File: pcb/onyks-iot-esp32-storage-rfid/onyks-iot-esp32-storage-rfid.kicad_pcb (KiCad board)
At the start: 4 copper layers, 79.5 x 45.5 mm, 22 parts, among them J1 Conn_01x02_Pin, J2 Conn_01x06_Pin, J3 Conn_02x05_Top_Bottom, J5 Conn_01x03_Pin, J6 Conn_01x01_Pin, Q1 SS8050, Q2 SS8050, SW3 SW_Push, SW4 SW_Push, U1 ESP32-WROOM-32D, U2 TLV75733PDBV

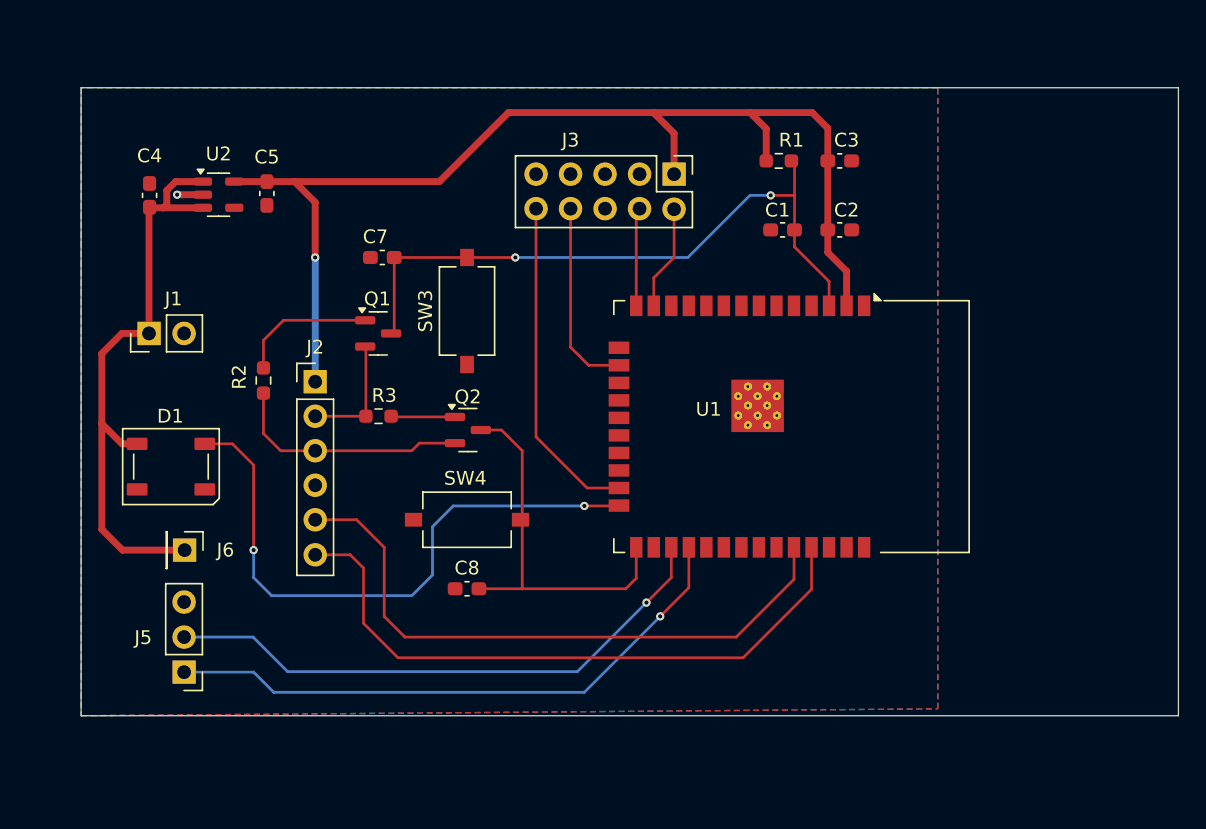
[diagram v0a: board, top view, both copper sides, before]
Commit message: PCB gotowe do review
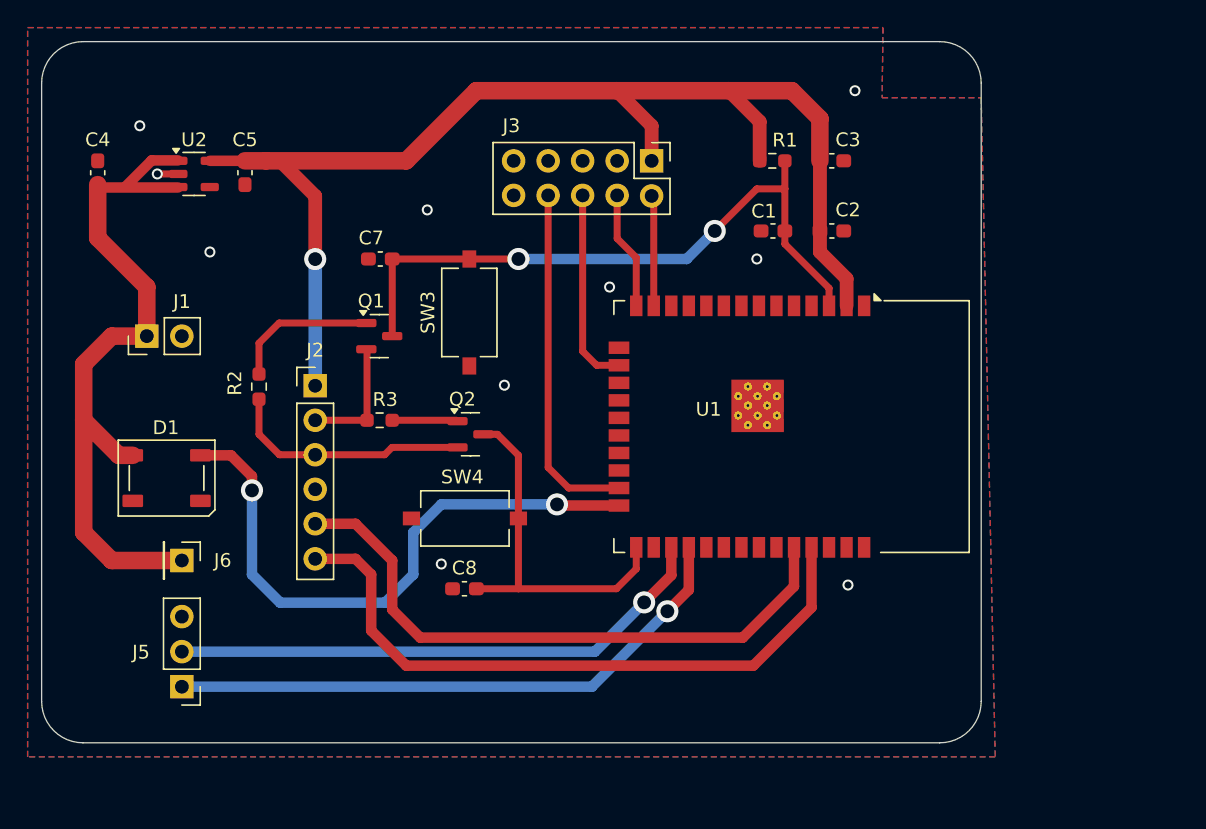
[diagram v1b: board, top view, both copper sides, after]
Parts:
- moved C4 4.10 mm to (110.7, 95.9)
- moved U2 2.33 mm to (117.7, 95.9)
- moved C5 2.19 mm to (121.4, 95.9)
- moved J3 1.89 mm to (150.9, 95.0)
- moved J5 1.07 mm to (116.8, 133.1)
- moved D1 0.89 mm to (115.7, 118.0)
- moved J6 0.78 mm to (116.8, 124.0)
- moved C1 0.70 mm to (159.7, 100.1)
- moved C2 0.57 mm to (163.9, 100.1)
- moved C3 0.57 mm to (163.9, 95.0)
- moved R2 0.55 mm to (122.4, 111.4)
- moved R1 0.47 mm to (159.6, 95.0)
- moved Q2 0.36 mm to (137.7, 114.8)
- moved R3 0.30 mm to (131.2, 113.8)
- moved J2 0.29 mm to (126.5, 111.3)
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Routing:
- net VCC: track 43.7 -> 52.8 mm
- net VDD33: track 83.2 -> 92.0 mm
- net /ESP32/RXD: track 41.4 -> 39.8 mm
- net /ESP32/MTDI: track 7.14 -> 8.57 mm
- net /ESP32/MTDO: track 24.1 -> 25.5 mm
- net /ESP32/PROGRAM_TXD: track 46.5 -> 47.6 mm
- net /ESP32/IO0: track 27.4 -> 26.6 mm
- net Net-(Q1-B): track 9.98 -> 10.6 mm
- net /ESP32/PROGRAM_RXD: track 45.2 -> 44.6 mm
- net /ESP32/TXD: track 43.2 -> 42.7 mm
- net /ESP32/EN: track 47.5 -> 48.0 mm
- net GND: track 1.86 -> 1.53 mm, vias 1 -> 10
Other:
- board size 79.5 x 45.5 mm -> 68.1 x 50.8 mm

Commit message: projekt PCB v2
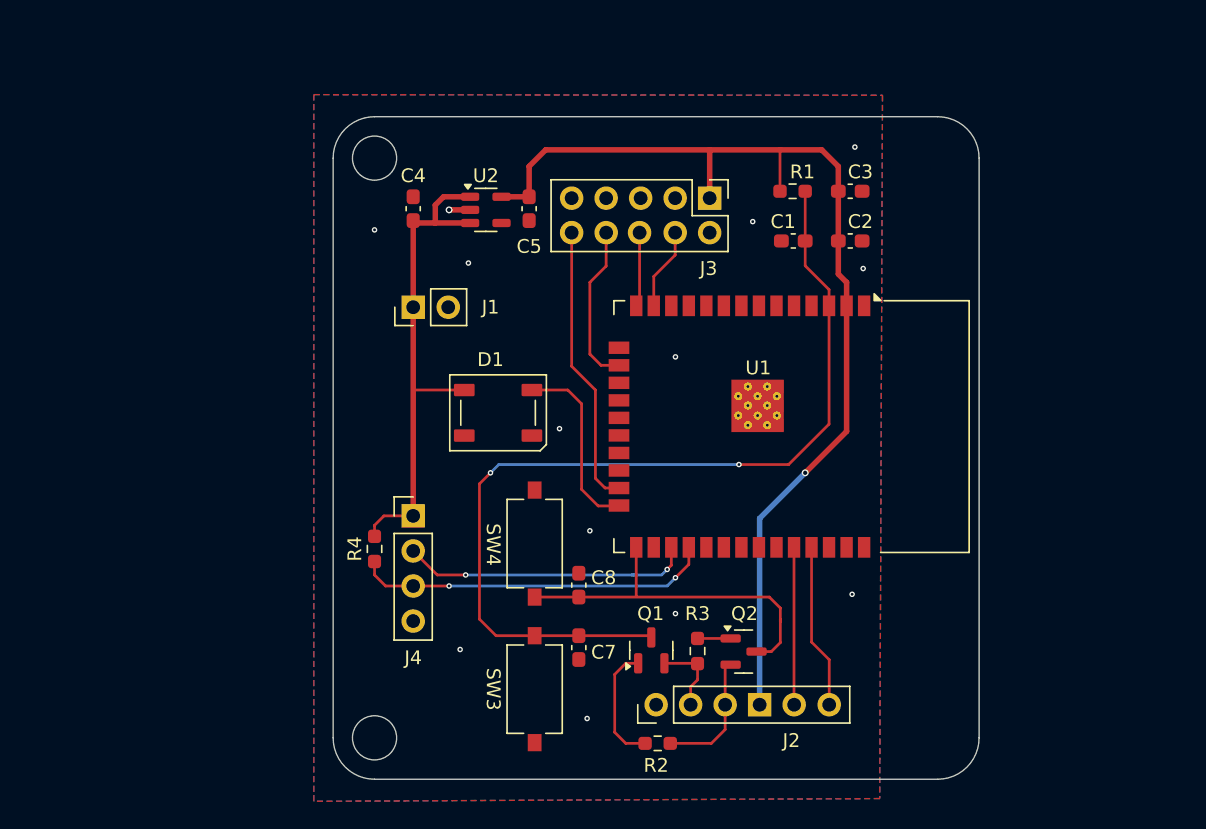
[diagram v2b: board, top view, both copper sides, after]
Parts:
- removed J5: Conn_01x03_Pin, Connector_PinHeader_2.54mm:PinHeader_1x03_P2.54mm_Vertical
- removed J6: Conn_01x01_Pin, Connector_PinHeader_2.54mm:PinHeader_1x01_P2.54mm_Vertical
- added J4: Conn_01x04_Pin, Connector_PinHeader_2.54mm:PinHeader_1x04_P2.54mm_Vertical, F.Cu at (133.6, 120.7)
- added R4: 10k, Resistor_SMD:R_0603_1608Metric_Pad0.98x0.95mm_HandSolder, F.Cu at (130.8, 123.1)
- moved R2 38.8 mm to (151.3, 137.2), turned to 180 degrees
- moved J2 33.8 mm to (151.2, 134.4), turned to 90 degrees
- moved C7 31.6 mm to (145.6, 130.3), turned to 90 degrees
- moved Q1 30.1 mm to (150.8, 130.5), turned to 90 degrees
- moved R3 28.5 mm to (154.2, 130.5), turned to 90 degrees
- moved SW3 27.7 mm to (142.4, 133.3)
- moved Q2 25.3 mm to (157.5, 130.6)
- moved D1 24.5 mm to (139.8, 113.2)
- moved C4 23.0 mm to (133.6, 98.5)
- moved U2 21.3 mm to (138.9, 98.5)
- moved C5 20.8 mm to (142.0, 98.5)
- moved J1 19.4 mm to (133.6, 105.6)
- moved C8 8.29 mm to (145.6, 125.7), turned to -90 degrees
- moved SW4 5.37 mm to (142.4, 122.7), turned to -90 degrees
- moved J3 5.00 mm to (155.1, 97.7)
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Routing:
- net /ESP32/PROGRAM_TXD: track 47.6 -> 11.9 mm
- net /ESP32/PROGRAM_RXD: track 44.6 -> 11.4 mm
- net /ESP32/LED: track 43.7 -> 13.4 mm, vias 2 -> 0
- net /ESP32/EN: track 48.0 -> 67.3 mm
- net /ESP32/RXD: track 39.8 -> 21.2 mm, vias 1 -> 2
- net /ESP32/TXD: track 42.7 -> 26.0 mm, vias 1 -> 2
- net VDD33: track 92.0 -> 76.0 mm
- net VCC: track 52.8 -> 37.0 mm
- net /ESP32/DTR: track 17.8 -> 9.19 mm
- net /ESP32/MTDO: track 25.5 -> 20.5 mm
- net /ESP32/MTDI: track 8.57 -> 5.06 mm
- net /ESP32/RTS: track 8.85 -> 5.56 mm
- net /ESP32/MTCK: track 14.3 -> 11.7 mm
- net Net-(Q2-B): track 4.66 -> 2.40 mm
- net /ESP32/MTMS: track 7.85 -> 5.98 mm
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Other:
- board size 68.1 x 50.8 mm -> 46.8 x 48 mm
